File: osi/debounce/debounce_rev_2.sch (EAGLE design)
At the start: 33 parts, among them IC1 74LS14D

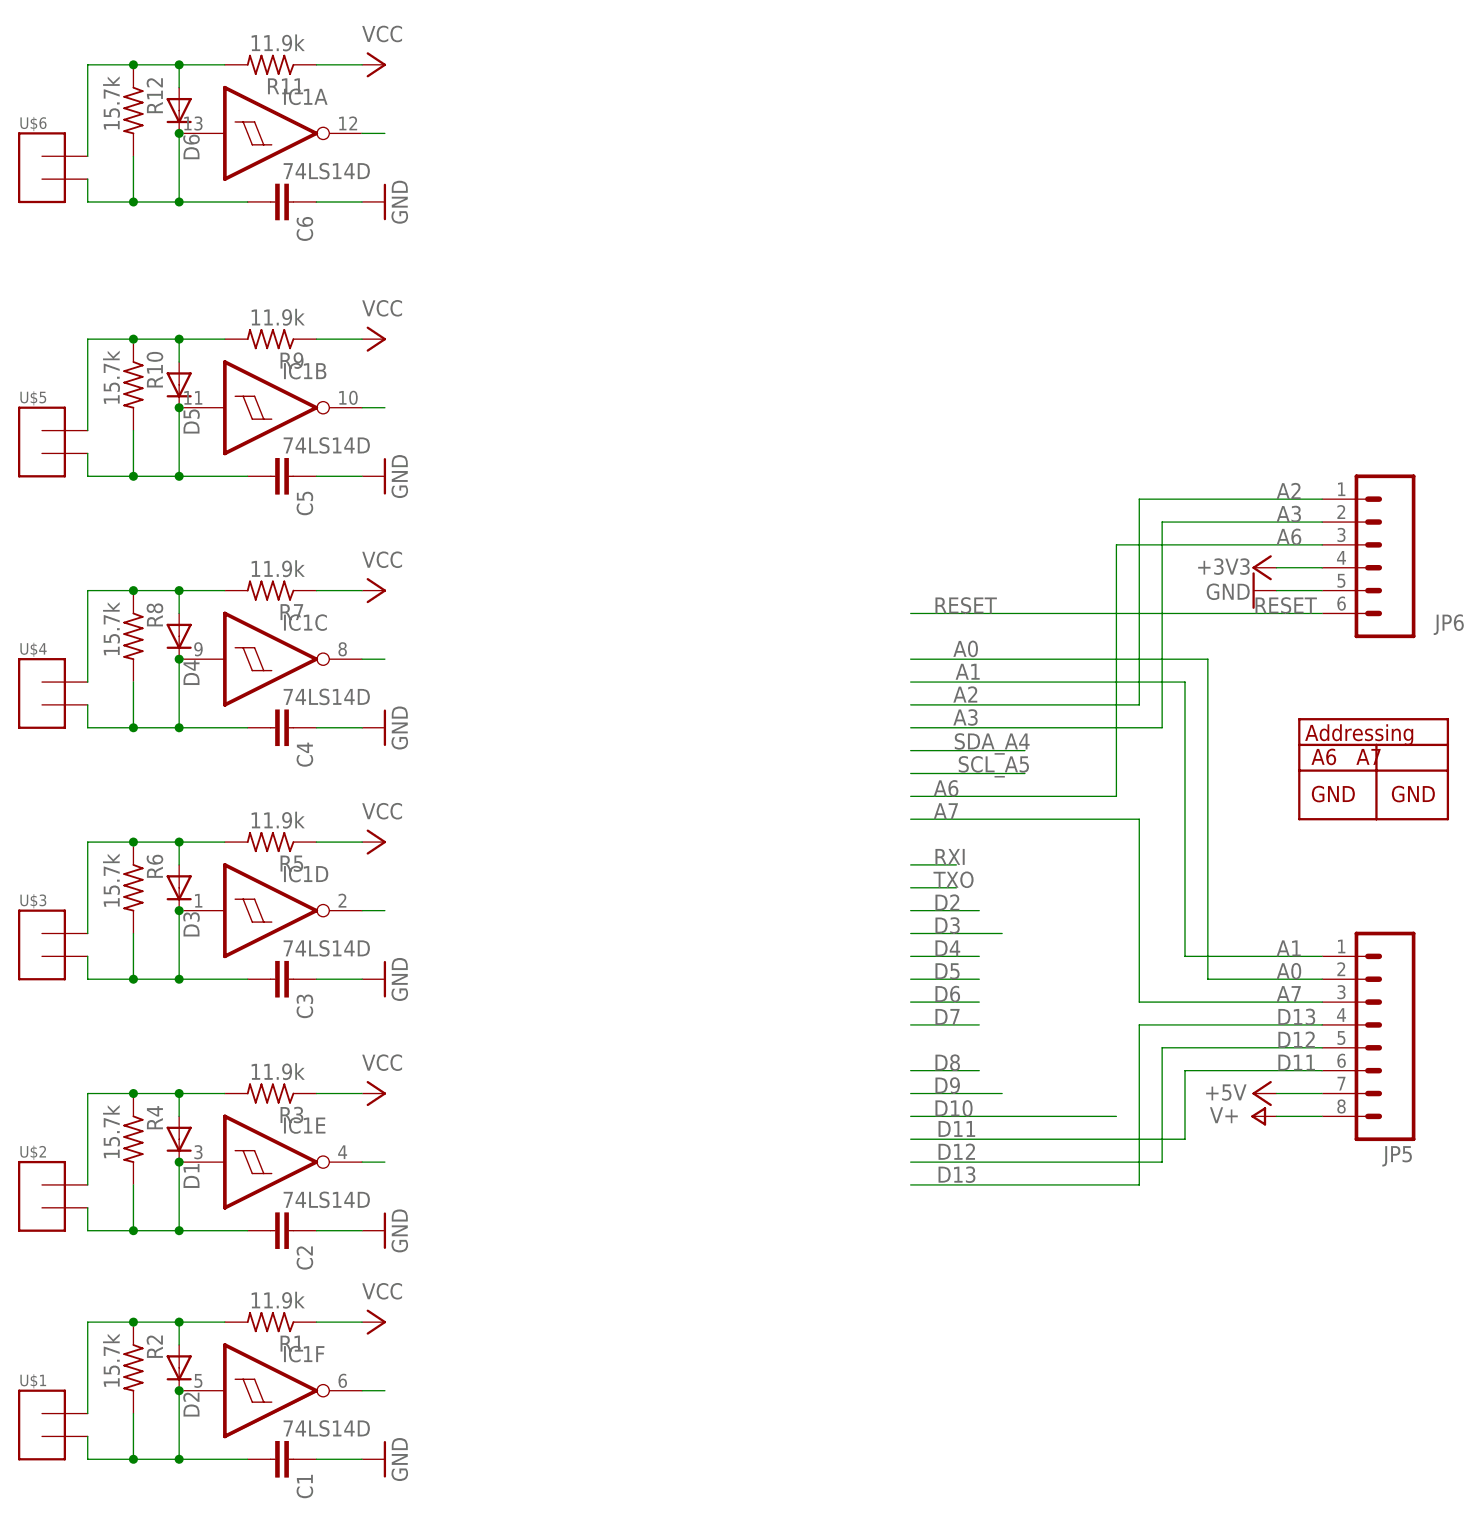
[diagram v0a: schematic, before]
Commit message: Furby work
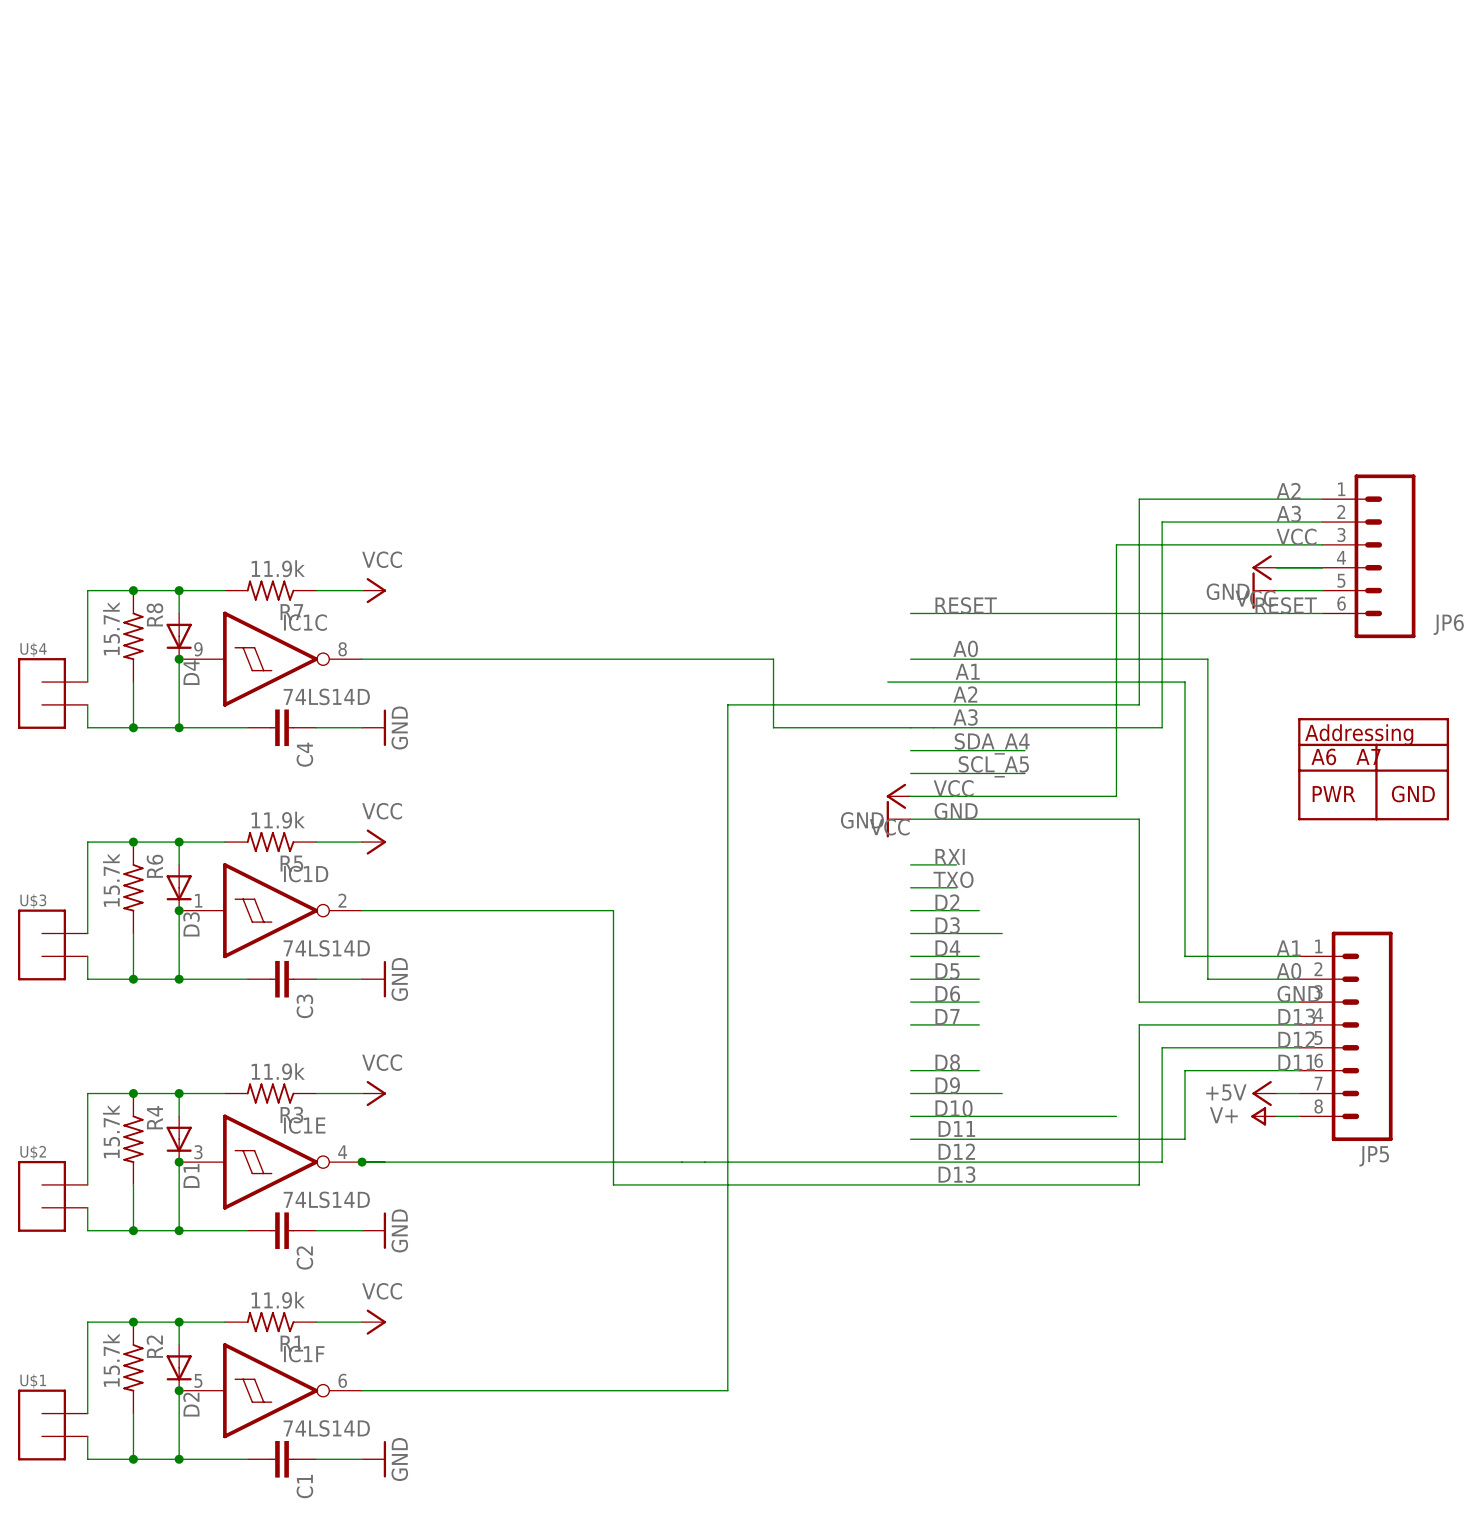
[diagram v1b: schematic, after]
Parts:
- removed C5, C6: (no value), SparkFun:CAPPTH
- removed D5, D6: (no value), diode:DIODE-D-2.5
- removed R10, R12: 15.7k, adafruit:R-US_0204/2V
- removed R11, R9: 11.9k, adafruit:R-US_0204/2V
- removed U$5, U$6: TERMINAL2, _my-parts:TERMINAL2
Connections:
- removed net +3V3: JP6.4
- removed net A6: JP6.3
- removed net A7: JP5.3
- removed net N$12: IC1C.O
- removed net N$13: D5.A, R10.1, R9.2, U$5.P$1
- removed net N$14: C5.2, D5.C, IC1B.I, R10.2, U$5.P$2
- removed net N$15: IC1B.O
- removed net N$16: D6.A, R11.2, R12.1, U$6.P$1
- removed net N$17: C6.2, D6.C, IC1A.I, R12.2, U$6.P$2
- removed net N$18: IC1A.O
- removed net N$5: IC1E.O
- removed net N$8: IC1F.O
- removed net N$9: IC1D.O
- net A2: now also IC1F.O
- net A3: now also IC1C.O
- net D12: now also IC1E.O
- net D13: now also IC1D.O
- net GND: now also JP5.3; no longer C5.1, C6.1
- net VCC: now also JP6.3, JP6.4; no longer R11.1, R9.1
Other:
- moved on the sheet: JP5
